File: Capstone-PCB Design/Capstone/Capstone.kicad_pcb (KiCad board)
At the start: 2 copper layers, 1 part

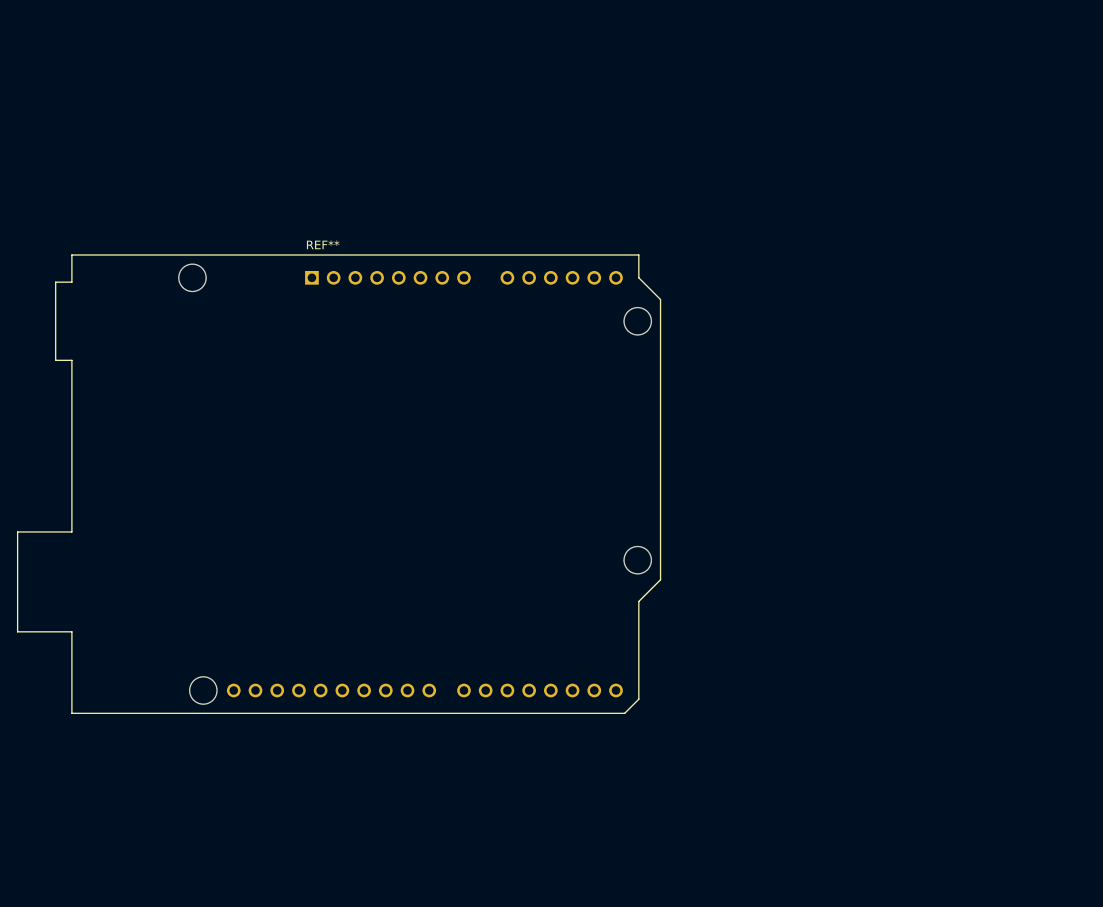
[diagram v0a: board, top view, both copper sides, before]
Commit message: PCB Design simulated w/ no errors
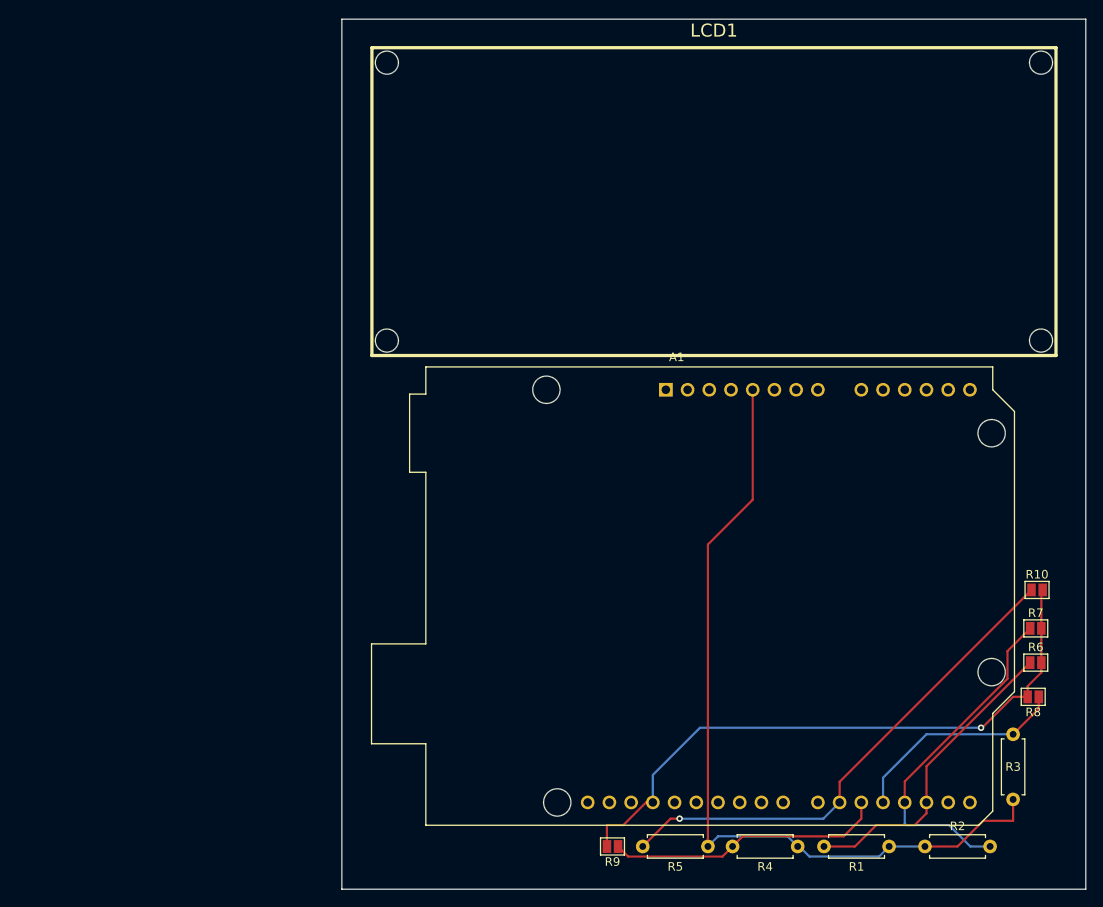
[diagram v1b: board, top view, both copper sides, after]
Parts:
- removed REF**: Arduino_UNO_R3_WithMountingHoles, Module:Arduino_UNO_R3_WithMountingHoles
- added A1: Arduino_UNO_R3, Module:Arduino_UNO_R3_WithMountingHoles, F.Cu at (124.9, 85.1)
- added LCD1: ~, Library:LCD-16x2, F.Cu at (130.5, 63.1)
- added R1: 5k, Resistor_THT:R_Axial_DIN0207_L6.3mm_D2.5mm_P7.62mm_Horizontal, F.Cu at (151.0, 138.5)
- added R10: R_Variable, Jumper:SolderJumper-2_P1.3mm_Open_Pad1.0x1.5mm, F.Cu at (168.3, 108.5)
- added R2: 5k, Resistor_THT:R_Axial_DIN0207_L6.3mm_D2.5mm_P7.62mm_Horizontal, F.Cu at (155.2, 138.5)
- added R3: 5k, Resistor_THT:R_Axial_DIN0207_L6.3mm_D2.5mm_P7.62mm_Horizontal, F.Cu at (165.5, 133.0)
- added R4: 5k, Resistor_THT:R_Axial_DIN0207_L6.3mm_D2.5mm_P7.62mm_Horizontal, F.Cu at (140.3, 138.5)
- added R5: 5k, Resistor_THT:R_Axial_DIN0207_L6.3mm_D2.5mm_P7.62mm_Horizontal, F.Cu at (129.8, 138.5)
- added R6: R_Variable, Jumper:SolderJumper-2_P1.3mm_Open_Pad1.0x1.5mm, F.Cu at (168.2, 117.0)
- added R7: R_Variable, Jumper:SolderJumper-2_P1.3mm_Open_Pad1.0x1.5mm, F.Cu at (168.2, 113.0)
- added R8: R_Variable, Jumper:SolderJumper-2_P1.3mm_Open_Pad1.0x1.5mm, F.Cu at (167.8, 121.0)
- added R9: R_Variable, Jumper:SolderJumper-2_P1.3mm_Open_Pad1.0x1.5mm, F.Cu at (118.7, 138.5)
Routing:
- net Net-(A1-+5V): track 0.00 -> 97.0 mm
- net Net-(LCD1-4): track 0.00 -> 73.0 mm, vias 0 -> 1
- net Net-(A1-D6): track 0.00 -> 59.3 mm, vias 0 -> 1
- net Net-(A1-D3): track 0.00 -> 40.0 mm
- net Net-(A1-D2): track 0.00 -> 36.2 mm
- net Net-(A1-D5): track 0.00 -> 32.7 mm
- net Net-(A1-D4): track 0.00 -> 25.8 mm
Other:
- board outline added: 87 x 101.8 mm
- rule pad_to_mask_clearance: 0 -> 0.0508
